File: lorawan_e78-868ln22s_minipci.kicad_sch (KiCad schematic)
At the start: 20 parts, among them Con1 MiniPci, Con2 TC2050-IDC-NL, P1 RF2-03E-T-00-50-G, U1 DS18B20U, U2 TCN75A, U8 IP4220CZ6

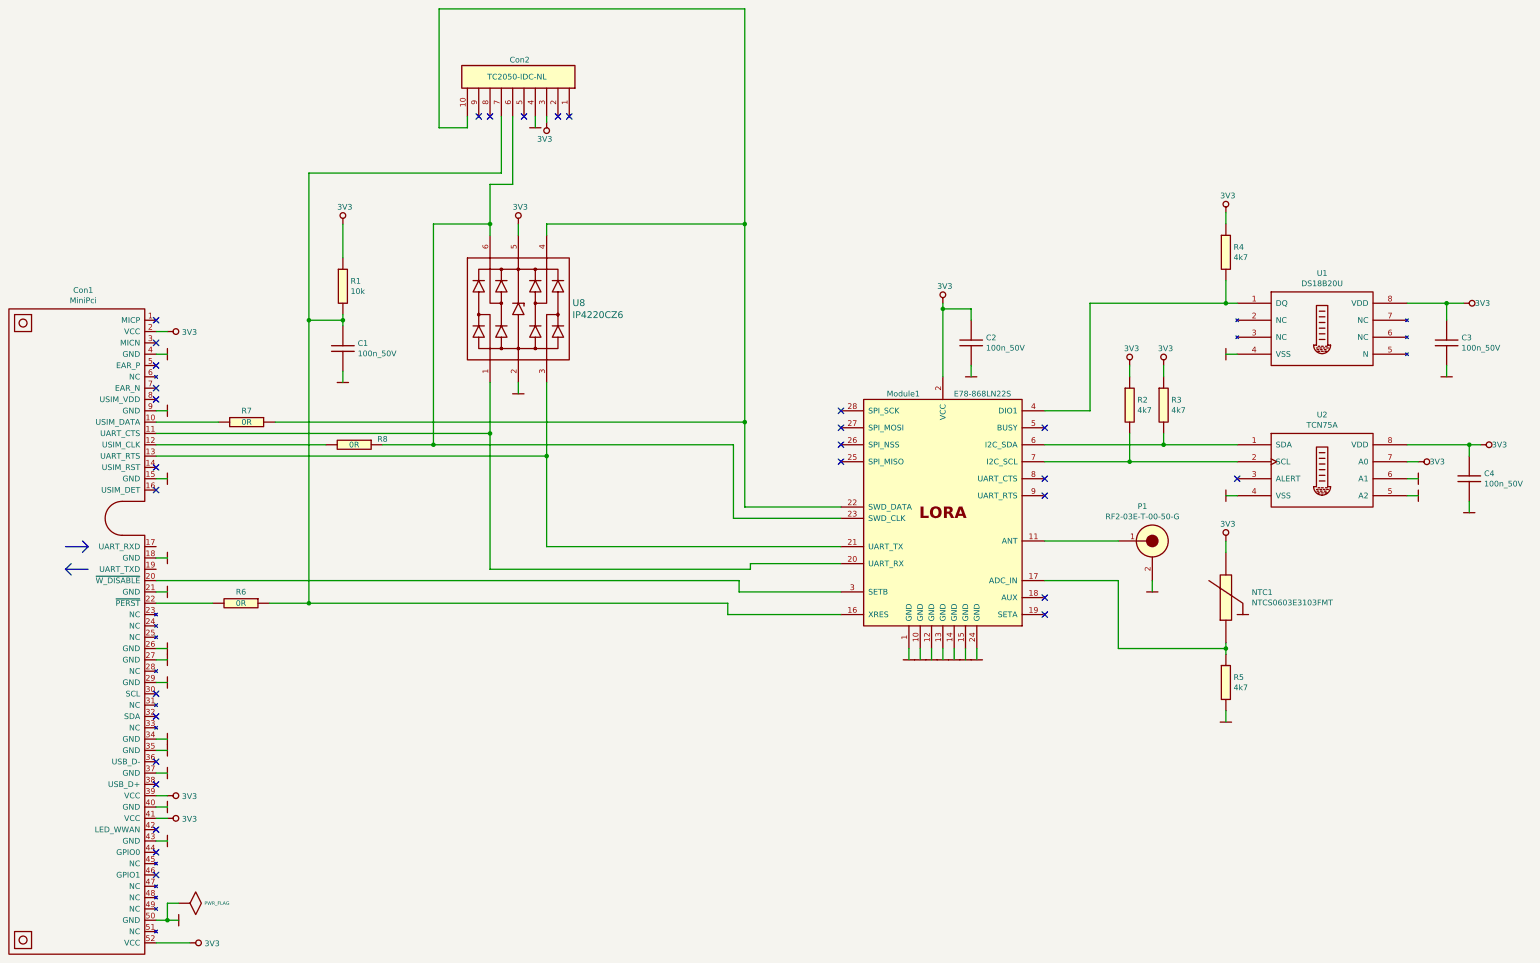
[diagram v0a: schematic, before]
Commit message: Corrected project
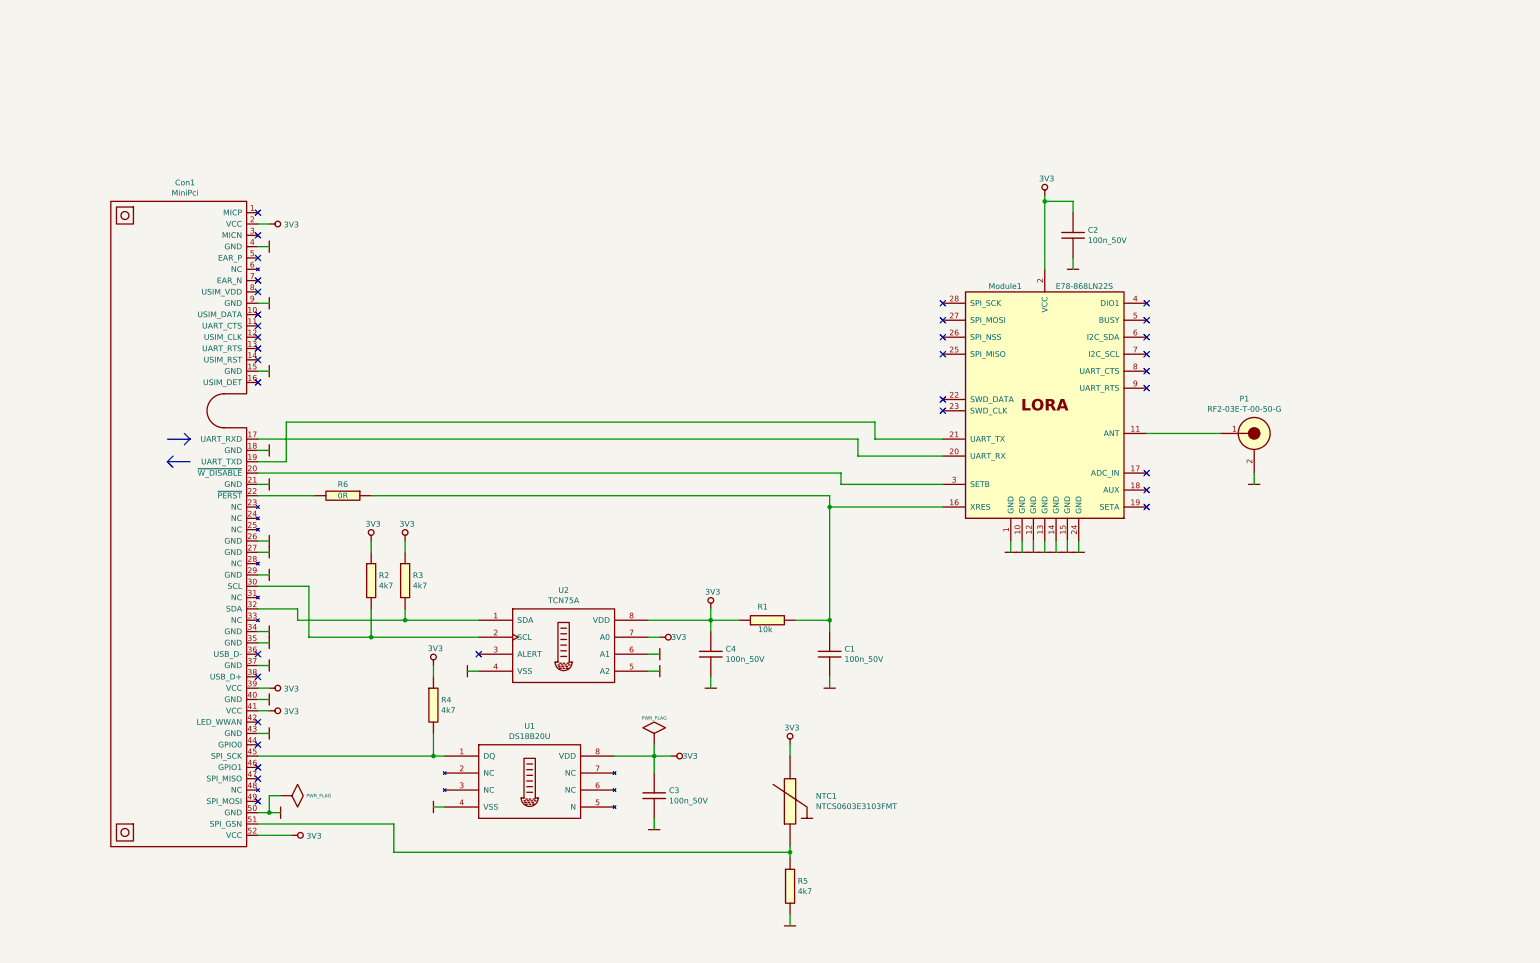
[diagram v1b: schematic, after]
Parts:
- removed Con2: TC2050-IDC-NL, Tag_Connectors:TC2050-IDC-NL, symbol Tag_Connectors:TC2050-IDC-NL
- removed R7, R8: 0R, Resistor_Smd_0603:0R_0603, symbol Resistors_Smd0603:0R
- removed U8: IP4220CZ6, ESD_Protectors:IP4220CZ6_SOT457, symbol esd_protectors:IP4220CZ6
- C1, C2, C3, C4: symbol Capacitors_Smd0603:100n_50V -> Capacitors_Smd0603:100n
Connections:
- net at Con1.11 (UART_CTS): no longer Module1.20 (UART_RX)
- net at Con1.13 (UART_RTS): no longer Module1.21 (UART_TX)
- net at Con1.17 (UART_RXD): now also Module1.20 (UART_RX)
- net at Con1.19 (UART_TXD): now also Module1.21 (UART_TX)
- net at Con1.30 (SCL): now also R2.2, U2.2 (SCL)
- net at Con1.32 (SDA): now also R3.2, U2.1 (SDA)
- net at Con1.45 (SPI_SCK): now also R4.2, U1.1 (DQ)
- net at Con1.51 (SPI_GSN): now also NTC1.1, R5.1
- now unconnected: Module1.17 (ADC_IN), Module1.4 (DIO1), Module1.6 (I2C_SDA), Module1.7 (I2C_SCL)
- no-connect marks 29 -> 34
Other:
- moved on the sheet: C1, C2, C3, C4, Module1, NTC1, P1, R1, R2, R3, R4, R5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
